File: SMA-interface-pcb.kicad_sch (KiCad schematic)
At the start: 9 parts, among them J1 Conn_Coaxial, J3 Conn_01x02_Pin, J4 USB_A_Stacked, J5 Conn_01x02_Pin, Q1 AO3400A, U1 EL817

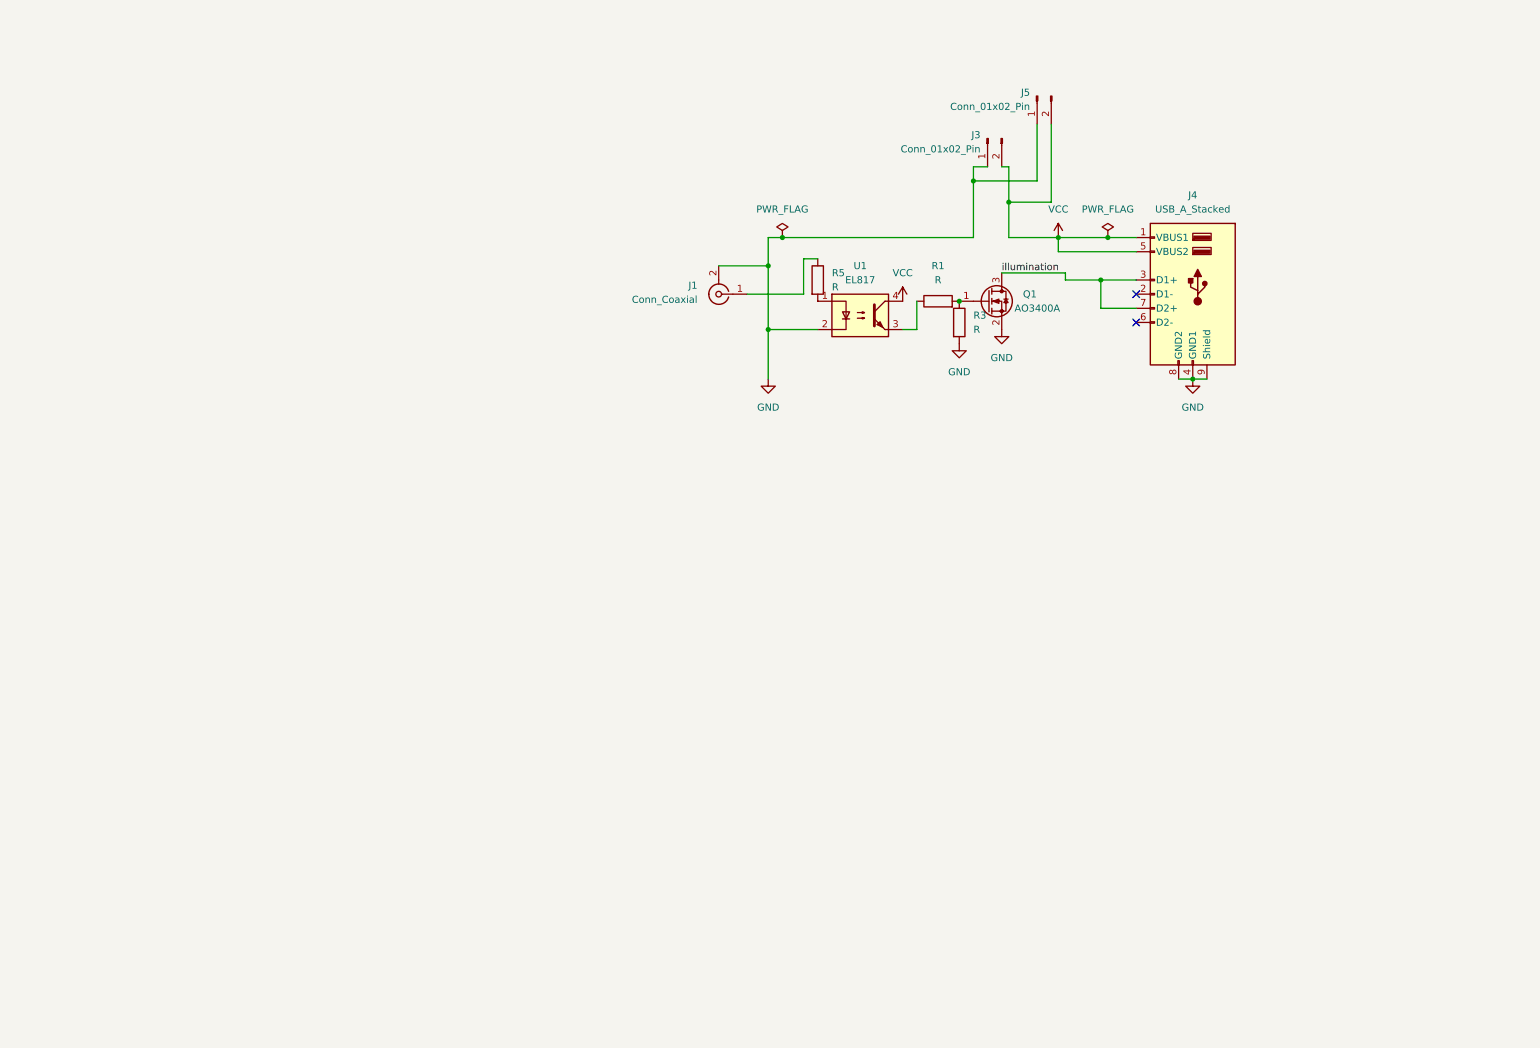
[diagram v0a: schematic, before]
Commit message: updated schematic to v0
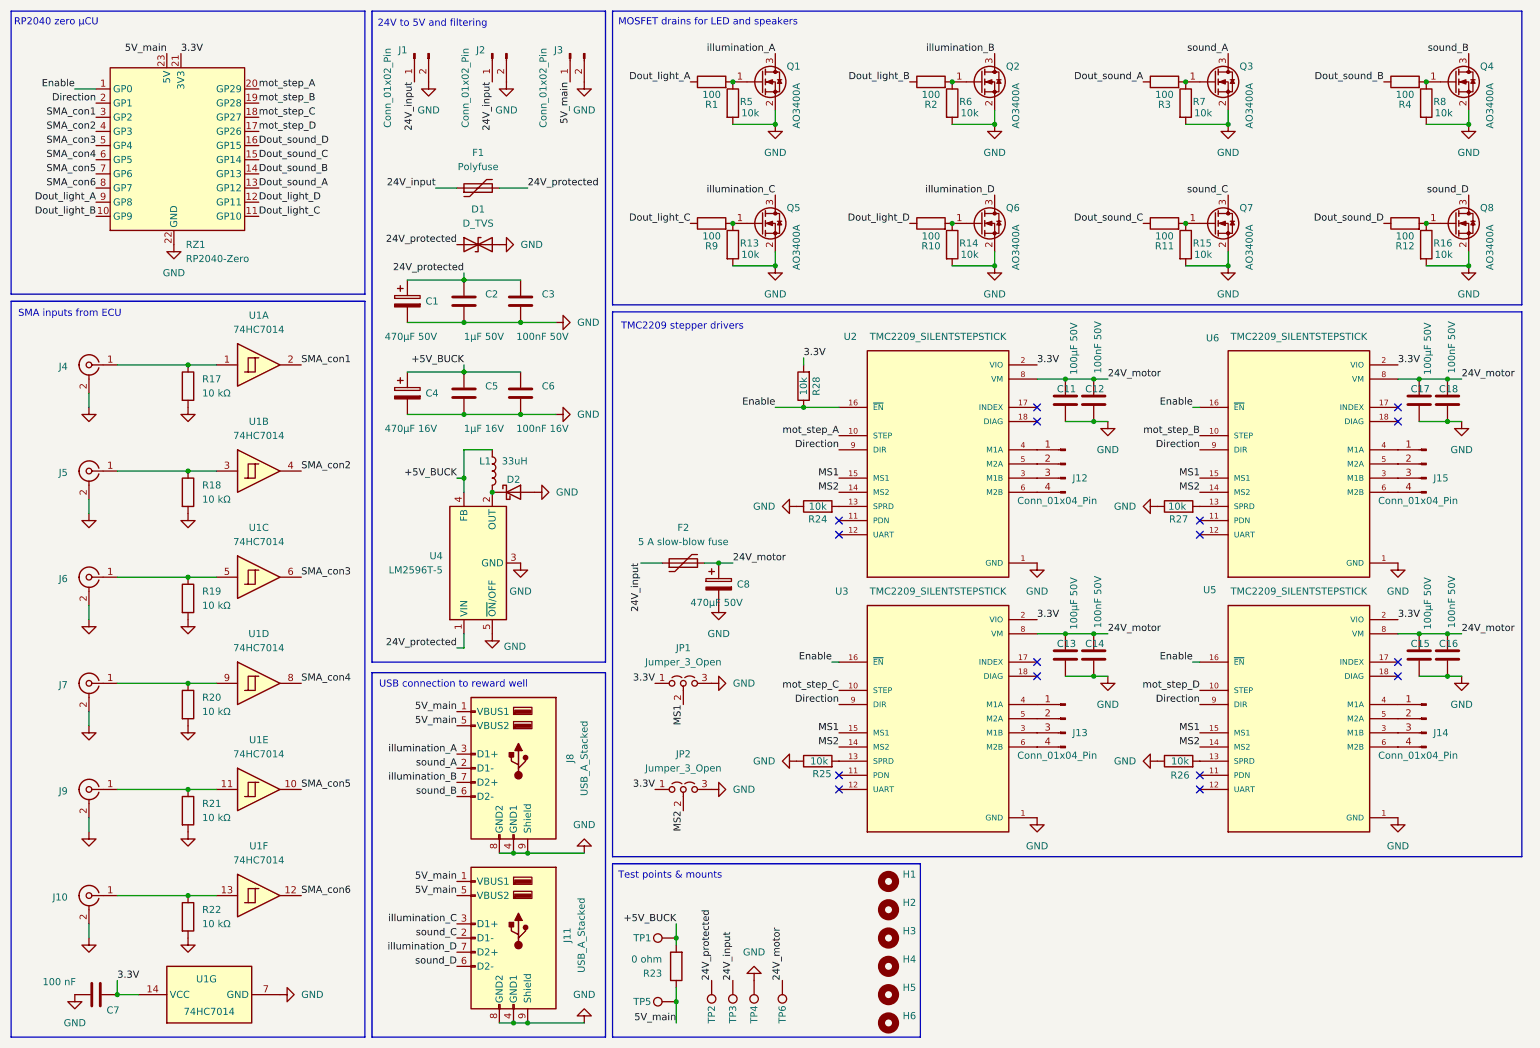
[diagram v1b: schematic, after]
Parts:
- removed J1: Conn_Coaxial, SMA:SMA_Amphenol_901-143_Horizontal, symbol Connector:Conn_Coaxial
- removed J4: USB_A_Stacked, Connector_USB:USB_A_Wuerth_61400826021_Horizontal_Stacked, symbol Connector:USB_A_Stacked
- removed J5: Conn_01x02_Pin, Connector_PinHeader_2.54mm:PinHeader_1x02_P2.54mm_Vertical, symbol Connector:Conn_01x02_Pin
- removed U1: EL817, Package_DIP:DIP-4_W7.62mm_SMDSocket_SmallPads, symbol Isolator:EL817
- added C1, C8: 470µF 50V, symbol Device:C_Polarized
- added C11, C13, C15, C17: 100µF 50V, symbol Device:C
- added C12, C14, C16, C18, C3: 100nF 50V, symbol Device:C
- added C2: 1µF 50V, symbol Device:C
- added C4: 470µF 16V, symbol Device:C_Polarized
- added C5: 1µF 16V, symbol Device:C
- added C6: 100nF 16V, symbol Device:C
- added C7: 100 nF, symbol Device:C
- added D1: D_TVS, symbol Device:D_TVS
- added D2: SS56B, Diode_SMD:D_3220_8050Metric_Pad2.65x5.15mm_HandSolder, symbol Device:D_Schottky
- added F1: Polyfuse, Fuse:fuse, symbol Device:Polyfuse
- added F2: 5 A slow-blow fuse, Fuse:fuse, symbol Device:Polyfuse
- added H1, H2, H3, H4, H5, H6: MountingHole, symbol Mechanical:MountingHole
- added J1, J2: Conn_01x02_Pin, Connector_Molex:Molex_Mini-Fit_Jr_5569-02A2_2x01_P4.20mm_Horizontal, symbol Connector:Conn_01x02_Pin
- added J10, J4, J5, J6, J7, J9: Conn_Coaxial, Connector_Coaxial:SMA_Amphenol_901-143_Horizontal, symbol Connector:Conn_Coaxial
- added J11, J8: USB_A_Stacked, Connector_USB:USB_A_Wuerth_61400826021_Horizontal_Stacked, symbol Connector:USB_A_Stacked
- added J12, J13, J14, J15: Conn_01x04_Pin, symbol Connector:Conn_01x04_Pin
- added JP1, JP2: Jumper_3_Open, Jumper:Jumper_Harwin_S1621_P10.9mm, symbol Jumper:Jumper_3_Open
- added L1: 33uH, symbol Device:L
- added Q2, Q3, Q4, Q5, Q6, Q7, Q8: AO3400A, Package_TO_SOT_SMD:SOT-23, symbol Transistor_FET:AO3400A
- added R10, R11, R12, R2, R4, R9: 100, Resistor_THT:R_Axial_DIN0207_L6.3mm_D2.5mm_P2.54mm_Vertical, symbol Device:R
- added R13, R14, R15, R16, R6, R7, R8: 10k, Resistor_THT:R_Axial_DIN0207_L6.3mm_D2.5mm_P2.54mm_Vertical, symbol Device:R
- added R17, R18, R19, R20, R21, R22: 10 kΩ, Resistor_THT:R_Axial_DIN0207_L6.3mm_D2.5mm_P2.54mm_Vertical, symbol Device:R
- added R23: 0 ohm, symbol Device:R
- added R24, R25, R26, R27, R28: 10k, symbol Device:R
- added RZ1: RP2040-Zero, RP2040:RP2040_Zero_Castellated, symbol RP2040_symbol:RP2040-Zero
- added TP1, TP2, TP3, TP4, TP5, TP6: TestPoint, symbol Connector:TestPoint
- added U1: 74HC7014, Package_SO:SOIC-14_3.9x8.7mm_P1.27mm, symbol 74xx:74HC7014
- added U2, U3, U5, U6: TMC2209_SILENTSTEPSTICK, TMC2209_SILENTSTEPSTICK:MODULE_TMC2209_SILENTSTEPSTICK, symbol NeuroACT:TMC2209_SILENTSTEPSTICK
- added U4: LM2596T-5, Package_TO_SOT_THT:TO-220-5_Vertical, symbol Regulator_Switching:LM2596T-5
- J3: footprint SMA:Molex_Mini-Fit_Jr_5569-02A2_2x01_P4.20mm_Horizontal -> Connector_Molex:Molex_Mini-Fit_Jr_5569-02A2_2x01_P4.20mm_Horizontal
- R1, R3: value R -> 100; footprint SMA:R_tht1270_smd3216 -> Resistor_THT:R_Axial_DIN0207_L6.3mm_D2.5mm_P2.54mm_Vertical
- R5: value R -> 10k; footprint SMA:R_tht1270_smd3216 -> Resistor_THT:R_Axial_DIN0207_L6.3mm_D2.5mm_P2.54mm_Vertical
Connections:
- net VCC is gone; now on net GND: J3.2 (Pin_2)
- net GND: now also R5.2, C1.2, C11.2, C12.2, C13.2, C14.2, C15.2, C16.2, C17.2, C18.2, C2.2, C3.2, C4.2, C5.2, C6.2, C7.1, C8.2, D1.2 (A2), D2.2 (A), J1.2 (Pin_2), J10.2 (Ext), J11.4 (GND1), J11.8 (GND2), J11.9 (Shield), J2.2 (Pin_2), J4.2 (Ext), J5.2 (Ext), J6.2 (Ext), J7.2 (Ext), J8.4 (GND1), J8.8 (GND2), J8.9 (Shield), J9.2 (Ext), JP1.3 (B), JP2.3 (B), Q2.2 (S), Q3.2 (S), Q4.2 (S), Q5.2 (S), Q6.2 (S), Q7.2 (S), Q8.2 (S), R13.2, R14.2, R15.2, R16.2, R17.2, R18.2, R19.2, R20.2, R21.2, R22.2, R24.1, R25.1, R26.1, R27.1, R6.2, R7.2, R8.2, RZ1.22 (GND), TP4.1, U1.7 (GND), U2.1 (GND), U2.7 (GND), U3.1 (GND), U3.7 (GND), U4.3 (GND), U4.5 (~{ON}/OFF), U5.1 (GND), U5.7 (GND), U6.1 (GND), U6.7 (GND); no longer J3.1 (Pin_1), R3.2
- net at R5.1: now also Q1.1 (G), R1.2
- net Dout_light_A: now reaches R1.1
- net Dout_light_A: now also RZ1.9 (GP8)
- net illumination renamed illumination_A
- net illumination_A: now also J8.3 (D1+)
- new net: Q4.1 (G), R4.2, R8.1
- new net: Q8.1 (G), R12.2, R16.1
- new net: J9.1 (In), R21.1, U1.11
- new net: Q2.1 (G), R2.2, R6.1
- new net: J5.1 (In), R18.1, U1.3
- new net: Q7.1 (G), R11.2, R15.1
- new net: Q6.1 (G), R10.2, R14.1
- new net: Q3.1 (G), R3.2, R7.1
- new net: R24.2, U2.13 (SPRD)
- new net: J12.3 (Pin_3), U2.3 (M1B)
- new net: J12.1 (Pin_1), U2.4 (M1A)
- new net: J12.2 (Pin_2), U2.5 (M2A)
- new net: J12.4 (Pin_4), U2.6 (M2B)
- new net: R27.2, U6.13 (SPRD)
- new net: J15.3 (Pin_3), U6.3 (M1B)
- new net: J15.1 (Pin_1), U6.4 (M1A)
- new net: J15.2 (Pin_2), U6.5 (M2A)
- new net: J15.4 (Pin_4), U6.6 (M2B)
- new net: R25.2, U3.13 (SPRD)
- new net: J10.1 (In), R22.1, U1.13
- new net: J7.1 (In), R20.1, U1.9
- new net: J6.1 (In), R19.1, U1.5
- new net: D2.1 (K), L1.1, U4.2 (OUT)
- new net: J13.1 (Pin_1), U3.4 (M1A)
- new net: J13.2 (Pin_2), U3.5 (M2A)
- new net: J13.3 (Pin_3), U3.3 (M1B)
- new net: J13.4 (Pin_4), U3.6 (M2B)
- new net: Q5.1 (G), R13.1, R9.2
- new net: R26.2, U5.13 (SPRD)
- new net: J4.1 (In), R17.1, U1.1
- new net: J14.3 (Pin_3), U5.3 (M1B)
- new net: J14.1 (Pin_1), U5.4 (M1A)
- new net: J14.2 (Pin_2), U5.5 (M2A)
- new net: J14.4 (Pin_4), U5.6 (M2B)
- new net +5V_BUCK: C4.1, C5.1, C6.1, L1.2, R23.2, TP1.1, U4.4 (FB)
- new net 24V_input: F1.1, F2.1, J1.1 (Pin_1), J2.1 (Pin_1), TP3.1
- new net 24V_motor: C11.1, C12.1, C13.1, C14.1, C15.1, C16.1, C17.1, C18.1, C8.1, F2.2, TP6.1, U2.8 (VM), U3.8 (VM), U5.8 (VM), U6.8 (VM)
- new net 24V_protected: C1.1, C2.1, C3.1, D1.1 (A1), F1.2, TP2.1, U4.1 (VIN)
- new net 3.3V: C7.2, JP1.1 (A), JP2.1 (A), R28.2, RZ1.21 (3V3), U1.14 (VCC), U2.2 (VIO), U3.2 (VIO), U5.2 (VIO), U6.2 (VIO)
- new net 5V_main: J11.1 (VBUS1), J11.5 (VBUS2), J3.1 (Pin_1), J8.1 (VBUS1), J8.5 (VBUS2), R23.1, RZ1.23 (5V), TP5.1
- new net Direction: RZ1.2 (GP1), U2.9 (DIR), U3.9 (DIR), U5.9 (DIR), U6.9 (DIR)
- new net Dout_light_B: R2.1, RZ1.10 (GP9)
- new net Dout_light_C: R9.1, RZ1.11 (GP10)
- new net Dout_light_D: R10.1, RZ1.12 (GP11)
- new net Dout_sound_A: R3.1, RZ1.13 (GP12)
- new net Dout_sound_B: R4.1, RZ1.14 (GP13)
- new net Dout_sound_C: R11.1, RZ1.15 (GP14)
- new net Dout_sound_D: R12.1, RZ1.16 (GP15)
- new net Enable: R28.1, RZ1.1 (GP0), U2.16 (~{EN}), U3.16 (~{EN}), U5.16 (~{EN}), U6.16 (~{EN})
- new net MS1: JP1.2 (C), U2.15 (MS1), U3.15 (MS1), U5.15 (MS1), U6.15 (MS1)
- new net MS2: JP2.2 (C), U2.14 (MS2), U3.14 (MS2), U5.14 (MS2), U6.14 (MS2)
- new net SMA_con1: RZ1.3 (GP2), U1.2
- new net SMA_con2: RZ1.4 (GP3), U1.4
- new net SMA_con3: RZ1.5 (GP4), U1.6
- new net SMA_con4: RZ1.6 (GP5), U1.8
- new net SMA_con5: RZ1.7 (GP6), U1.10
- new net SMA_con6: RZ1.8 (GP7), U1.12
- new net illumination_B: J8.7 (D2+), Q2.3 (D)
- new net illumination_C: J11.3 (D1+), Q5.3 (D)
- new net illumination_D: J11.7 (D2+), Q6.3 (D)
- new net mot_step_A: RZ1.20 (GP29), U2.10 (STEP)
- new net mot_step_B: RZ1.19 (GP28), U6.10 (STEP)
- new net mot_step_C: RZ1.18 (GP27), U3.10 (STEP)
- new net mot_step_D: RZ1.17 (GP26), U5.10 (STEP)
- new net sound_A: J8.2 (D1-), Q3.3 (D)
- new net sound_B: J8.6 (D2-), Q4.3 (D)
- new net sound_C: J11.2 (D1-), Q7.3 (D)
- new net sound_D: J11.6 (D2-), Q8.3 (D)
- no-connect marks 2 -> 16
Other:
- note added: "24V to 5V and filtering"
- note added: "MOSFET drains for LED and speakers"
- note added: "RP2040 zero µCU"
- note added: "SMA inputs from ECU"
- note added: "TMC2209 stepper drivers"
- note added: "Test points & mounts"
- note added: "USB connection to reward well"
- company: (none) -> NeuroACT lab, NCBS
- title: (none) -> SMA interface board
